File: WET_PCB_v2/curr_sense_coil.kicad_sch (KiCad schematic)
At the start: 0 parts

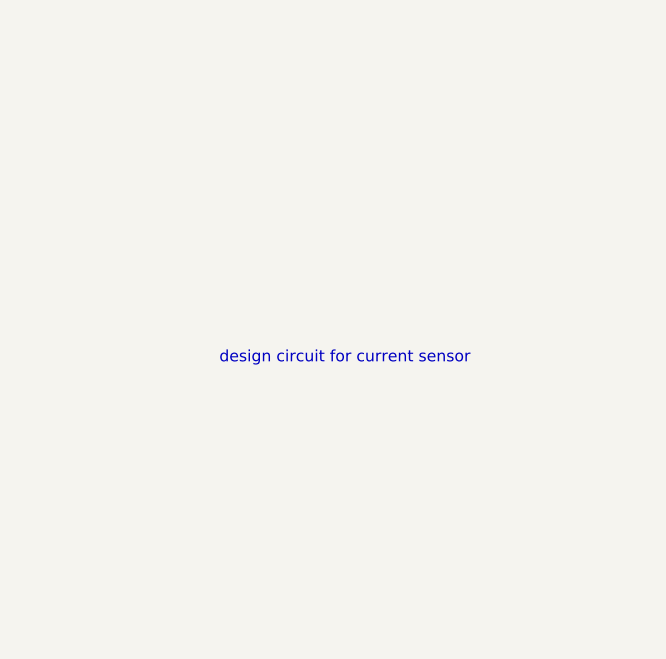
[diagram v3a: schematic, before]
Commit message: before i prob fuck up everything bc clearance
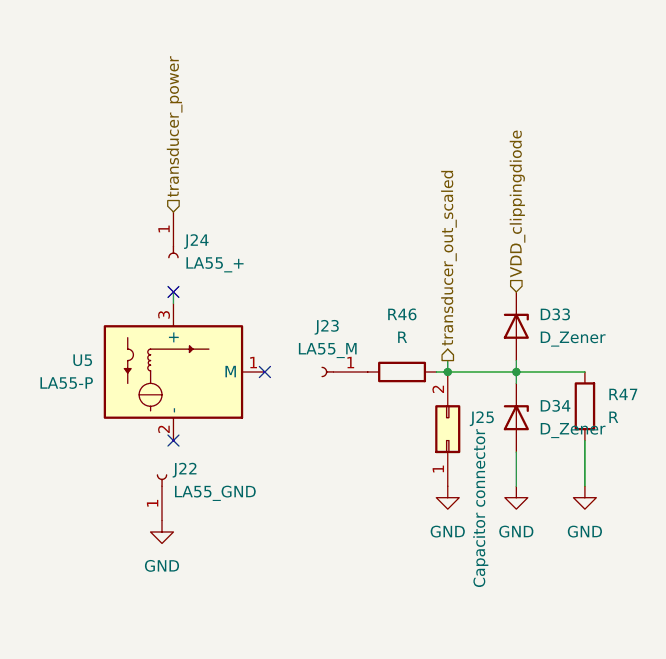
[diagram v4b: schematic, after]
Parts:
- added D33, D34: D_Zener, Diode_THT:D_DO-15_P2.54mm_Vertical_CathodeUp, symbol Device:D_Zener
- added J22: LA55_GND, Connector_PinSocket_2.54mm:PinSocket_1x01_P2.54mm_Horizontal, symbol Connector:Conn_01x01_Socket
- added J23: LA55_M, Connector_PinSocket_2.54mm:PinSocket_1x01_P2.54mm_Horizontal, symbol Connector:Conn_01x01_Socket
- added J24: LA55_+, Connector_PinSocket_2.54mm:PinSocket_1x01_P2.54mm_Horizontal, symbol Connector:Conn_01x01_Socket
- added J25: Capacitor connector, Connector_PinSocket_2.54mm:PinSocket_1x02_P2.54mm_Vertical, symbol Connector_Generic:Conn_02x01
- added R46, R47: R, Resistor_SMD:R_0805_2012Metric_Pad1.20x1.40mm_HandSolder, symbol Device:R
- added U5: LA55-P, Sensor_Current:LEM_LA25-P, symbol Sensor_Current:LA55-P
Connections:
- new net: J23.1 (Pin_1), R46.1
- new net GND: D34.2 (A), J22.1 (Pin_1), J25.1 (Pin_1), R47.1
- new net VDD_clippingdiode: D33.1 (K)
- new net transducer_out_scaled: D33.2 (A), D34.1 (K), J25.2 (Pin_2), R46.2, R47.2
- new net transducer_power: J24.1 (Pin_1)
- no-connect marks 0 -> 3
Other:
- note removed: "design circuit for current sensor"
